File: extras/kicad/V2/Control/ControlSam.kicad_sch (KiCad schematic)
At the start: 55 parts, among them J1 Ultrasonic Ranging, J2 Conn_01x05, J3 Output, J4 Input, J6 left, J7 right, J8 UEXT_Host, J9 Conn_01x07, P8 BeagleBone_Black_Header, P9 BeagleBone_Black_Header, U1 SparkFun-micromod, U2 MPU-6050, U3 CD4052B, U4 BNO085-breackout, U5 TJA1042T-3, U6 PCA9557PW

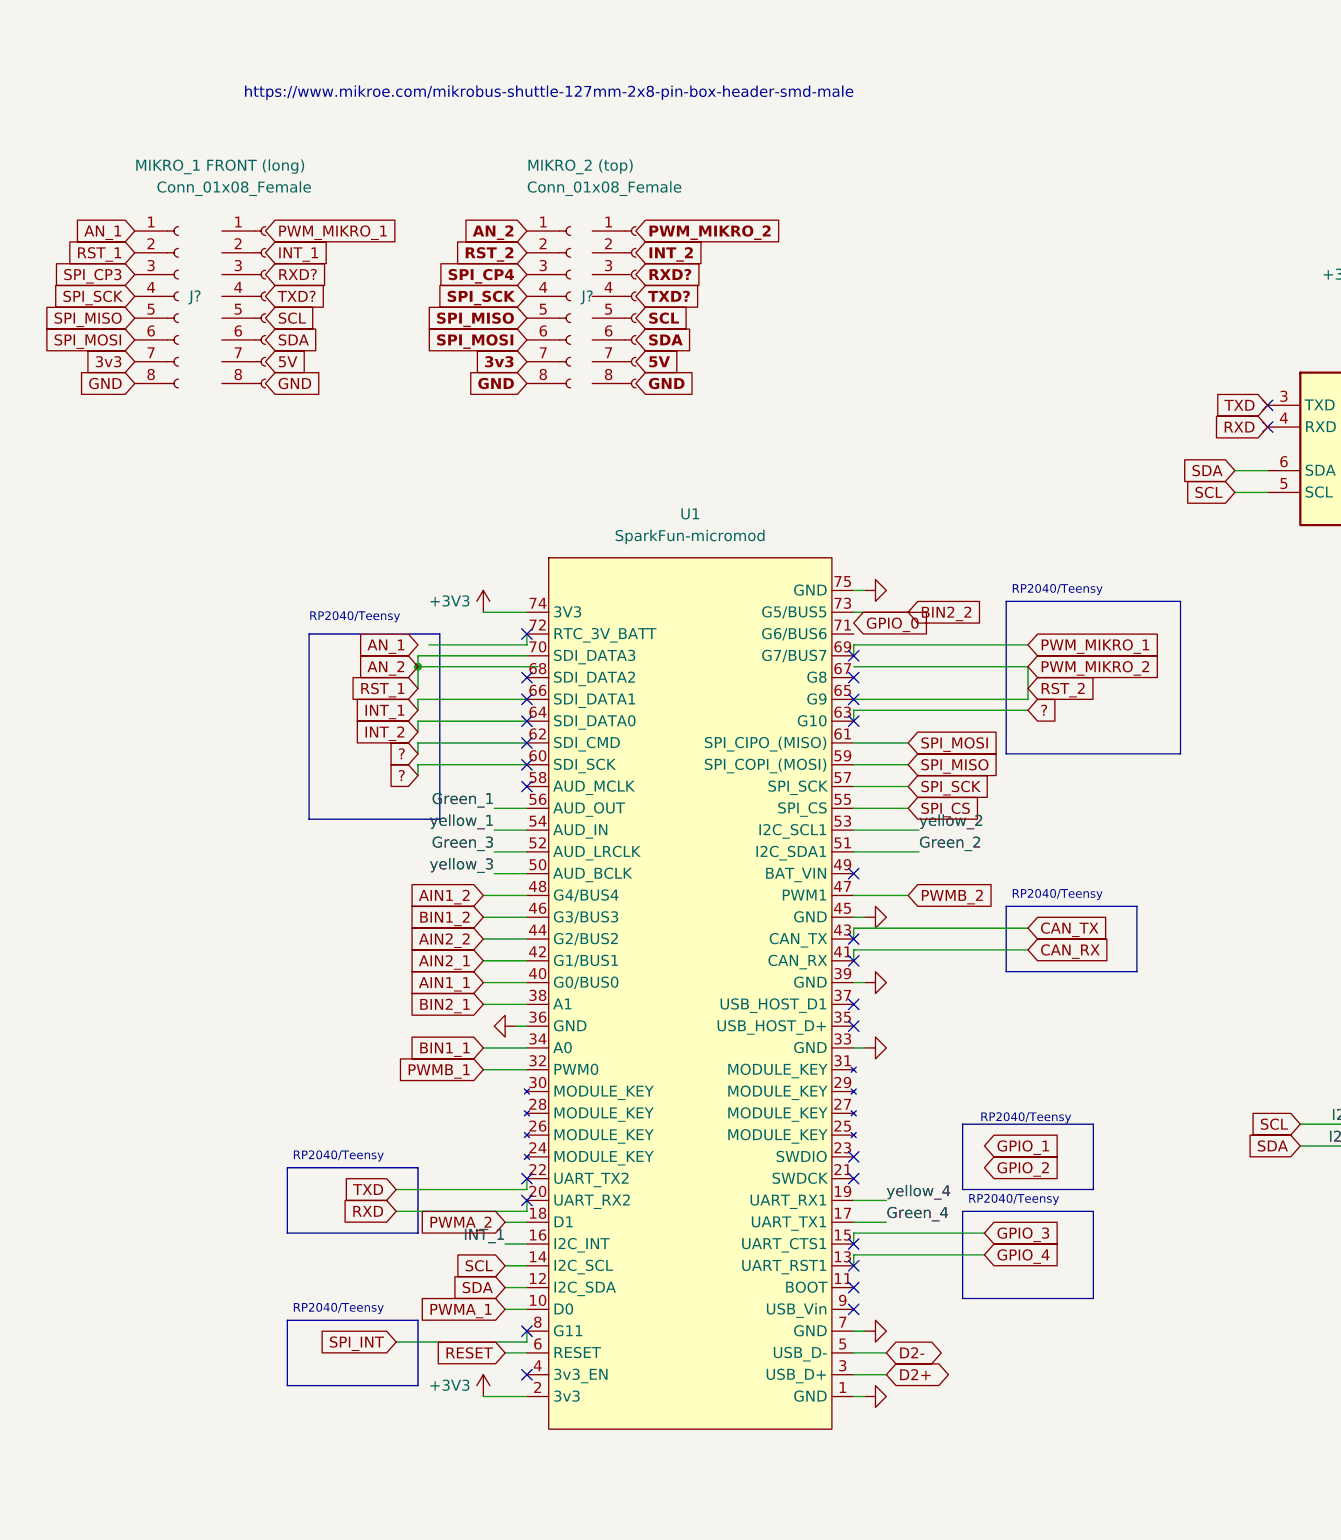
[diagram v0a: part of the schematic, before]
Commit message: Update ControlSam.kicad_sch
Tidying
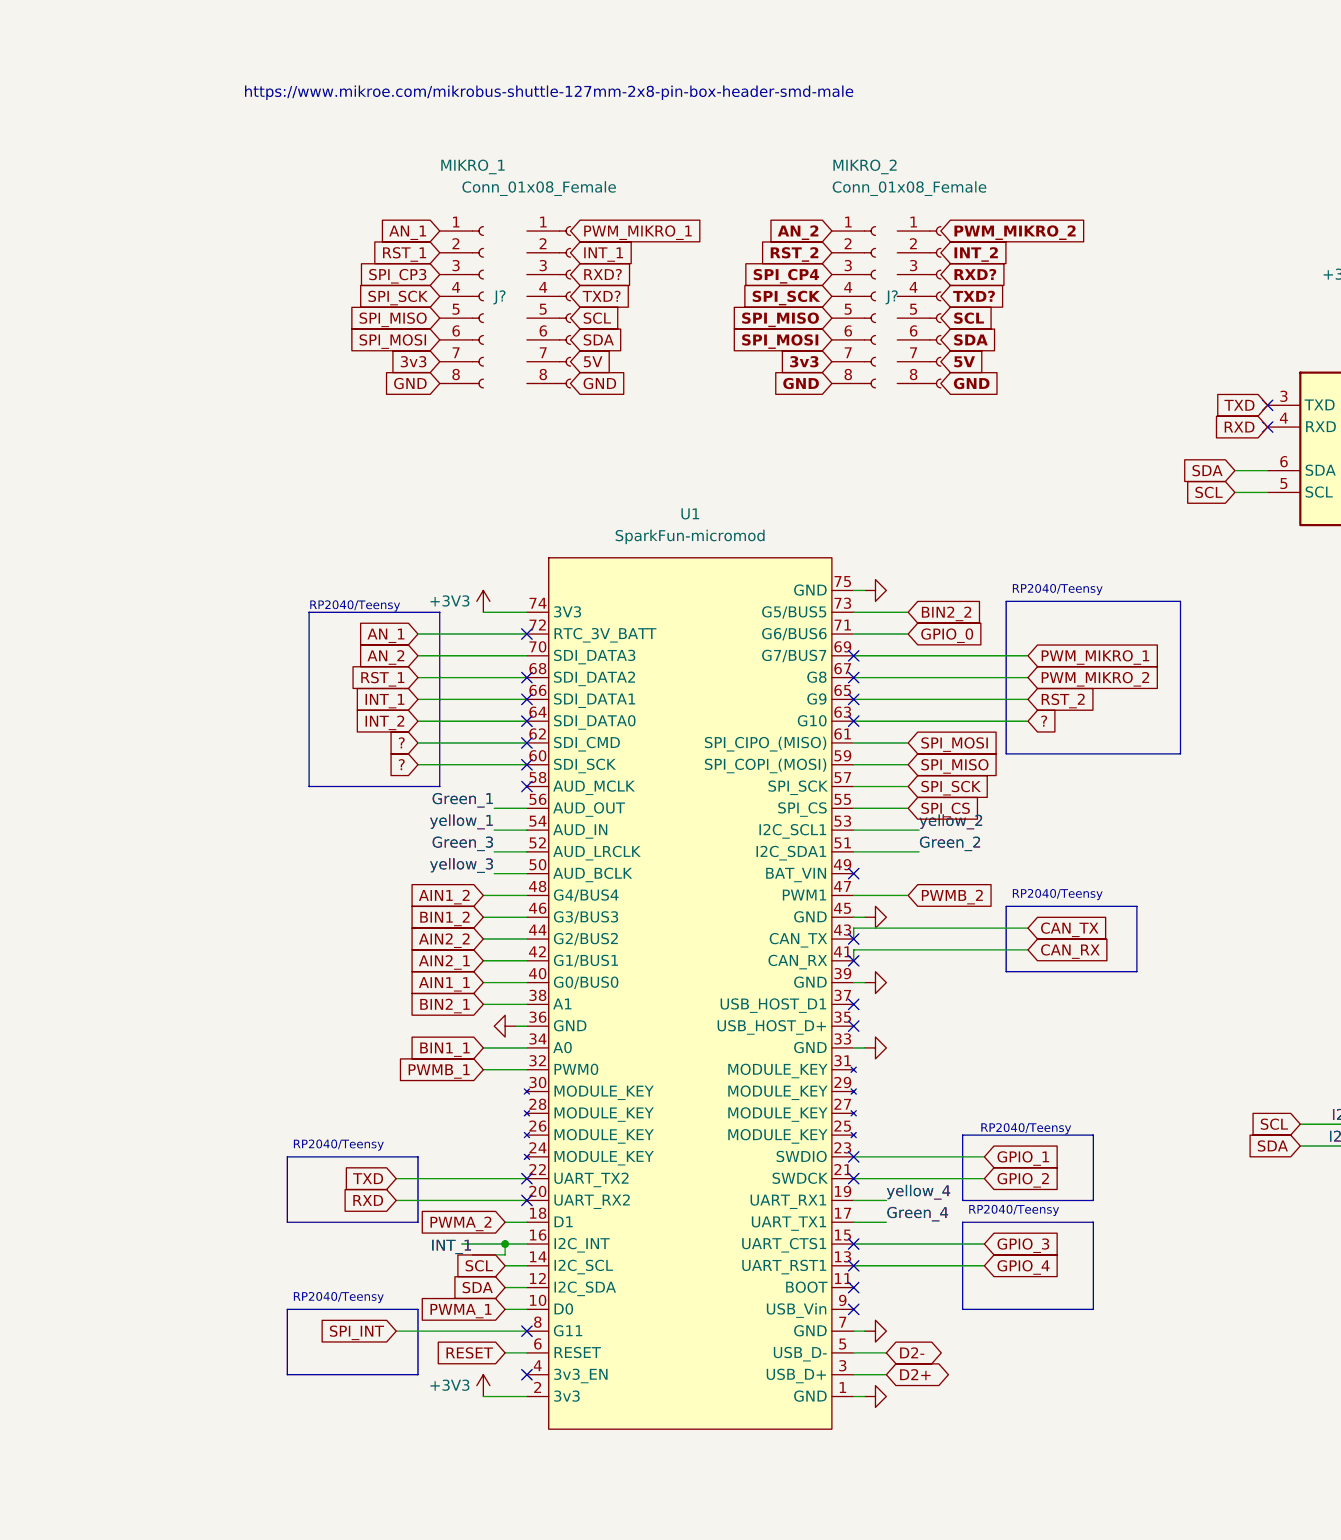
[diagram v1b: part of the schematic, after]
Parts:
- J?: value MIKRO_2 (top) -> MIKRO_2
- J?: value MIKRO_1 FRONT (long) -> MIKRO_1
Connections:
- net AN_1: now also U1.72 (RTC_3V_BATT)
- net AN_2: no longer J?.2 (Pin_2)
- net GPIO_0: now also U1.71 (G6/BUS6)
- net GPIO_1: now also U1.23 (SWDIO)
- net GPIO_2: now also U1.21 (SWDCK)
- net PWM_MIKRO_2: now also U1.67 (G8); no longer J?.2 (Pin_2), U1.65 (G9)
- net RST_1: now reaches U1.68 (SDI_DATA2)
- net RST_1: now also J?.2 (Pin_2)
- new net RST_2: J?.2 (Pin_2), U1.65 (G9)
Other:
- moved on the sheet: J?

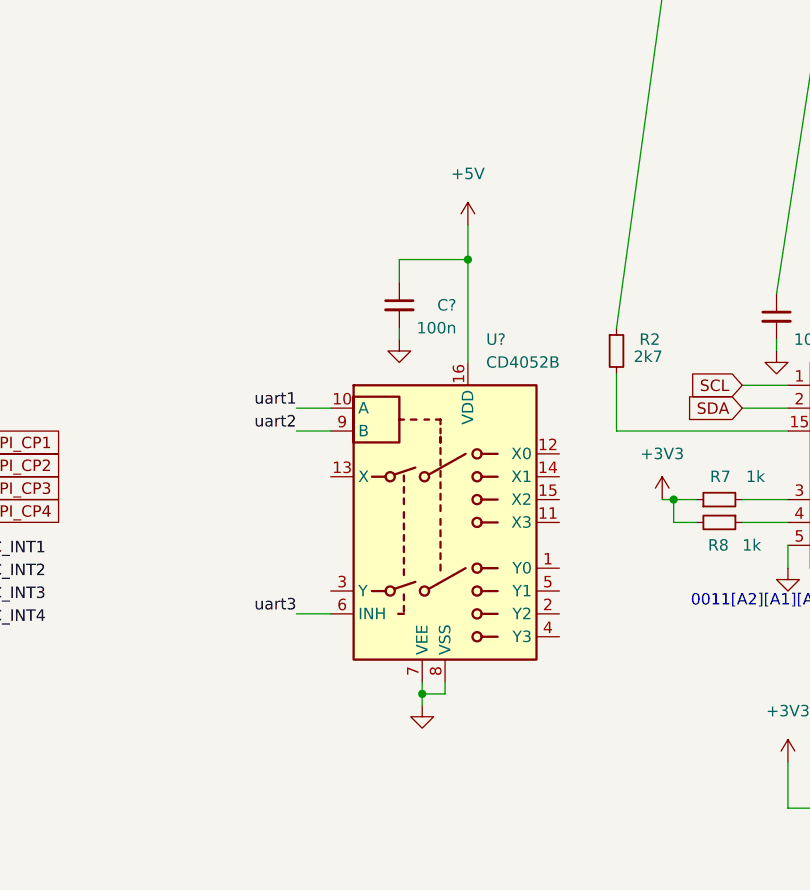
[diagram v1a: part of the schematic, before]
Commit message: Update ControlSam.kicad_sch
Sync
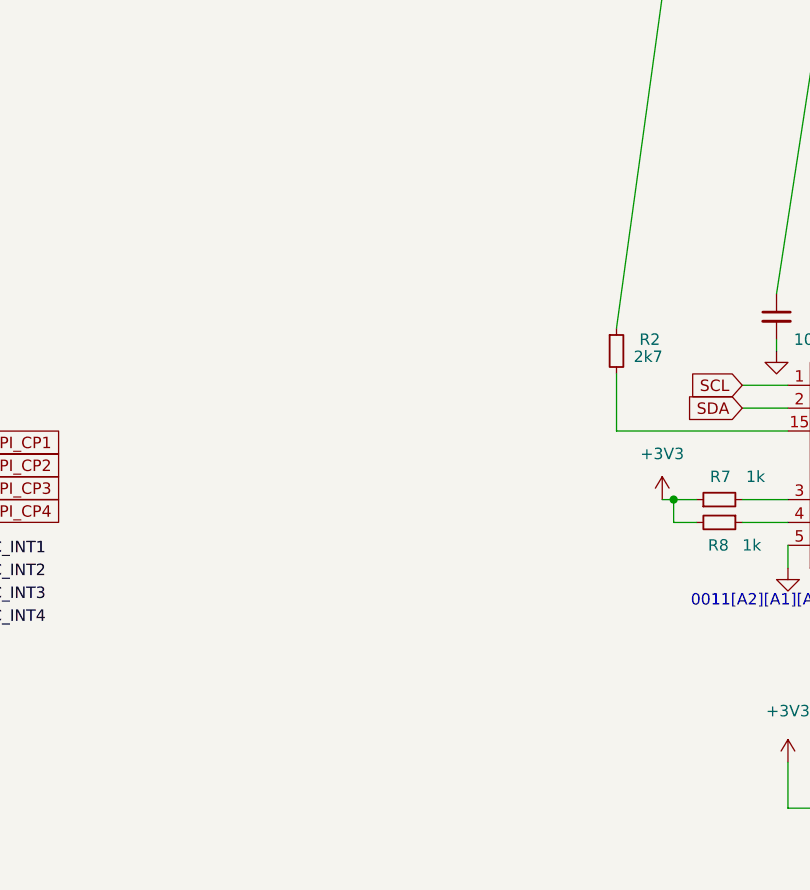
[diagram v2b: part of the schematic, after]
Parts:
- removed C?: 100n, Capacitor_SMD:C_0603_1608Metric_Pad1.08x0.95mm_HandSolder, symbol Device:C_Small
- removed U?: CD4052B, Package_SO:SOIC-16_3.9x9.9mm_P1.27mm, symbol Analog_Switch:CD4052B
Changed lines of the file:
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@@
   (junction (at 349.25 445.77) (diameter 0) (color 0 0 0 0)
   )
-  (junction (at 119.38 90.17) (diameter 0) (color 0 0 0 0)
-  )
   (junction (at 466.09 463.55) (diameter 0) (color 0 0 0 0)
   )
@@
   (junction (at 355.6 149.86) (diameter 0) (color 0 0 0 0)
   )
-  (junction (at 124.46 41.91) (diameter 0) (color 0 0 0 0)
-  )
   (junction (at 340.36 149.86) (diameter 0) (color 0 0 0 0)
   )
@@
     (stroke (width 0) (type solid))
   )
-  (wire (pts (xy 105.41 58.42) (xy 109.22 58.42))
-    (stroke (width 0) (type default))
-  )
   (wire (pts (xy 232.41 208.28) (xy 226.06 208.28))
     (stroke (width 0) (type default))
@@
     (stroke (width 0) (type default))
   )
-  (wire (pts (xy 121.92 88.9) (xy 121.92 90.17))
-    (stroke (width 0) (type default))
-  )
   (wire (pts (xy 59.69 219.71) (xy 63.5 219.71))
     (stroke (width 0) (type default))
@@
     (stroke (width 0) (type solid))
   )
-  (wire (pts (xy 116.84 49.53) (xy 116.84 50.8))
-    (stroke (width 0) (type default))
-  )
   (wire (pts (xy 160.02 102.87) (xy 172.72 102.87))
     (stroke (width 0) (type default))
@@
     (stroke (width 0) (type default))
   )
-  (wire (pts (xy 116.84 41.91) (xy 124.46 41.91))
-    (stroke (width 0) (type default))
-  )
   (wire (pts (xy 335.28 149.86) (xy 340.36 149.86))
     (stroke (width 0) (type default))
@@
     (stroke (width 0) (type default))
   )
-  (wire (pts (xy 105.41 60.96) (xy 109.22 60.96))
-    (stroke (width 0) (type default))
-  )
   (wire (pts (xy 574.04 -17.78) (xy 577.85 -17.78))
     (stroke (width 0) (type default))
@@
     (stroke (width 0) (type solid))
   )
-  (wire (pts (xy 119.38 90.17) (xy 119.38 91.44))
-    (stroke (width 0) (type default))
-  )
   (wire (pts (xy 233.68 128.27) (xy 231.14 128.27))
     (stroke (width 0) (type default))
   )
-  (wire (pts (xy 124.46 41.91) (xy 124.46 53.34))
-    (stroke (width 0) (type default))
-  )
   (wire (pts (xy 193.04 102.87) (xy 200.66 102.87))
     (stroke (width 0) (type default))
@@
     (stroke (width 0) (type default))
   )
-  (wire (pts (xy 116.84 41.91) (xy 116.84 44.45))
-    (stroke (width 0) (type default))
-  )
   (wire (pts (xy 321.31 -64.77) (xy 340.36 -64.77))
     (stroke (width 0) (type solid))
@@
     (stroke (width 0) (type solid))
   )
-  (wire (pts (xy 119.38 90.17) (xy 121.92 90.17))
-    (stroke (width 0) (type default))
-  )
   (wire (pts (xy 250.19 -21.59) (xy 269.24 -21.59))
     (stroke (width 0) (type solid))
@@
     (stroke (width 0) (type default))
   )
-  (wire (pts (xy 119.38 88.9) (xy 119.38 90.17))
-    (stroke (width 0) (type default))
-  )
   (wire (pts (xy 353.06 -54.61) (xy 372.11 -54.61))
     (stroke (width 0) (type solid))
@@
     (stroke (width 0) (type solid))
   )
-  (wire (pts (xy 124.46 38.1) (xy 124.46 41.91))
-    (stroke (width 0) (type default))
-  )
   (wire (pts (xy 58.42 229.87) (xy 63.5 229.87))
     (stroke (width 0) (type default))
@@
     (stroke (width 0) (type default))
   )
-  (wire (pts (xy 105.41 81.28) (xy 109.22 81.28))
-    (stroke (width 0) (type default))
-  )
   (wire (pts (xy 281.94 -59.69) (xy 300.99 -59.69))
     (stroke (width 0) (type solid))
@@
     (effects (font (size 1.27 1.27)) (justify left bottom))
   )
-  (label "uart3" (at 105.41 81.28 180) (fields_autoplaced)
-    (effects (font (size 1.27 1.27)) (justify right bottom))
-  )
   (label "CAN_H" (at 195.58 -21.59 0) (fields_autoplaced)
     (effects (font (size 1.27 1.27)) (justify left bottom))
@@
     (effects (font (size 1.27 1.27)) (justify right bottom))
   )
-  (label "uart2" (at 105.41 60.96 180) (fields_autoplaced)
-    (effects (font (size 1.27 1.27)) (justify right bottom))
-  )
   (label "cc2" (at 361.95 453.39 0) (fields_autoplaced)
     (effects (font (size 1.27 1.27)) (justify left bottom))
@@
     (effects (font (size 1.27 1.27)) (justify left bottom))
   )
-  (label "uart1" (at 105.41 58.42 180) (fields_autoplaced)
-    (effects (font (size 1.27 1.27)) (justify right bottom))
-  )
   (label "CAN_STB" (at 160.02 -13.97 180) (fields_autoplaced)
     (effects (font (size 1.27 1.27)) (justify right bottom))
@@
     )
   )
-  (symbol (lib_id "power:+5V") (at 124.46 38.1 0) (unit 1)
-    (in_bom yes) (on_board yes) (dnp no) (fields_autoplaced)
-    (property "Reference" "#PWR?" (at 124.46 41.91 0)
-      (effects (font (size 1.27 1.27)) hide)
-    )
-    (property "Value" "+5V" (at 124.46 32.385 0)
-      (effects (font (size 1.27 1.27)))
-    )
-    (property "Footprint" "" (at 124.46 38.1 0)
-      (effects (font (size 1.27 1.27)) hide)
-    )
-    (property "Datasheet" "" (at 124.46 38.1 0)
-      (effects (font (size 1.27 1.27)) hide)
-    )
-    (pin "1")
-    (instances
-      (project "ControlSam"
-        (path "/9c56e35b-b900-4603-b0fe-ca83857f3d6c"
-          (reference "#PWR?") (unit 1)
-        )
-      )
-    )
-  )
   (symbol (lib_id "Mechanical:MountingHole_Pad") (at 308.61 38.1 0) (unit 1)
     (in_bom no) (on_board yes) (dnp no)
@@
     )
   )
-  (symbol (lib_id "Analog_Switch:CD4052B") (at 121.92 71.12 0) (unit 1)
-    (in_bom yes) (on_board yes) (dnp no) (fields_autoplaced)
-    (property "Reference" "U?" (at 126.4794 50.8 0)
-      (effects (font (size 1.27 1.27)) (justify left))
-    )
-    (property "Value" "CD4052B" (at 126.4794 53.34 0)
-      (effects (font (size 1.27 1.27)) (justify left))
-    )
-    (property "Footprint" "Package_SO:SOIC-16_3.9x9.9mm_P1.27mm" (at 125.73 90.17 0)
-      (effects (font (size 1.27 1.27)) (justify left) hide)
-    )
-    (property "Datasheet" "http://www.ti.com/lit/ds/symlink/cd4052b.pdf" (at 121.412 66.04 0)
-      (effects (font (size 1.27 1.27)) hide)
-    )
-    (property "LCSC" "C6521" (at 121.92 71.12 0)
-      (effects (font (size 1.27 1.27)) hide)
-    )
-    (pin "1")
-    (pin "10")
-    (pin "11")
-    (pin "12")
-    (pin "13")
-    (pin "14")
-    (pin "15")
-    (pin "16")
-    (pin "2")
-    (pin "3")
-    (pin "4")
-    (pin "5")
-    (pin "6")
-    (pin "7")
-    (pin "8")
-    (pin "9")
-    (instances
-      (project "ControlSam"
-        (path "/9c56e35b-b900-4603-b0fe-ca83857f3d6c"
-          (reference "U?") (unit 1)
-        )
-      )
-    )
-  )
   (symbol (lib_id "power:GND") (at 102.87 232.41 90) (unit 1)
     (in_bom yes) (on_board yes) (dnp no) (fields_autoplaced)
@@
     )
   )
-  (symbol (lib_id "Device:C_Small") (at 116.84 46.99 0) (mirror y) (unit 1)
-    (in_bom yes) (on_board yes) (dnp no)
-    (property "Reference" "C?" (at 123.19 46.99 0)
-      (effects (font (size 1.27 1.27)) (justify left))
-    )
-    (property "Value" "100n" (at 123.19 49.53 0)
-      (effects (font (size 1.27 1.27)) (justify left))
-    )
-    (property "Footprint" "Capacitor_SMD:C_0603_1608Metric_Pad1.08x0.95mm_HandSolder" (at 116.84 46.99 0)
-      (effects (font (size 1.27 1.27)) hide)
-    )
-    (property "Datasheet" "~" (at 116.84 46.99 0)
-      (effects (font (size 1.27 1.27)) hide)
-    )
-    (property "LCSC" "C14663" (at 116.84 46.99 0)
-      (effects (font (size 1.27 1.27)) hide)
-    )
-    (pin "1")
-    (pin "2")
-    (instances
-      (project "ControlSam"
-        (path "/9c56e35b-b900-4603-b0fe-ca83857f3d6c"
-          (reference "C?") (unit 1)
-        )
-      )
-    )
-  )
-  (symbol (lib_id "power:GND") (at 119.38 91.44 0) (mirror y) (unit 1)
-    (in_bom yes) (on_board yes) (dnp no) (fields_autoplaced)
-    (property "Reference" "#PWR?" (at 119.38 97.79 0)
-      (effects (font (size 1.27 1.27)) hide)
-    )
-    (property "Value" "GND" (at 119.38 96.52 0)
-      (effects (font (size 1.27 1.27)) hide)
-    )
-    (property "Footprint" "" (at 119.38 91.44 0)
-      (effects (font (size 1.27 1.27)) hide)
-    )
-    (property "Datasheet" "" (at 119.38 91.44 0)
-      (effects (font (size 1.27 1.27)) hide)
-    )
-    (pin "1")
-    (instances
-      (project "ControlSam"
-        (path "/9c56e35b-b900-4603-b0fe-ca83857f3d6c"
-          (reference "#PWR?") (unit 1)
-        )
-      )
-    )
-  )
   (symbol (lib_id "Sensor_Motion:MPU-6050") (at 337.82 173.99 0) (unit 1)
     (in_bom yes) (on_board yes) (dnp no) (fields_autoplaced)
@@
         )
       )
-    )
-  )
-  (symbol (lib_id "power:GND") (at 116.84 50.8 0) (mirror y) (unit 1)
-    (in_bom yes) (on_board yes) (dnp no) (fields_autoplaced)
-    (property "Reference" "#PWR?" (at 116.84 57.15 0)
-      (effects (font (size 1.27 1.27)) hide)
-    )
-    (property "Value" "GND" (at 116.84 55.88 0)
-      (effects (font (size 1.27 1.27)) hide)
-    )
-    (property "Footprint" "" (at 116.84 50.8 0)
-      (effects (font (size 1.27 1.27)) hide)
-    )
-    (property "Datasheet" "" (at 116.84 50.8 0)
-      (effects (font (size 1.27 1.27)) hide)
-    )
-    (pin "1")
-    (instances
-      (project "ControlSam"
-        (path "/9c56e35b-b900-4603-b0fe-ca83857f3d6c"
-          (reference "#PWR?") (unit 1)
-        )
-      )
